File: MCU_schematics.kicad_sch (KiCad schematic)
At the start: 39 parts, among them Q1 SS8050, Q2 SS8050, U7 CH340C

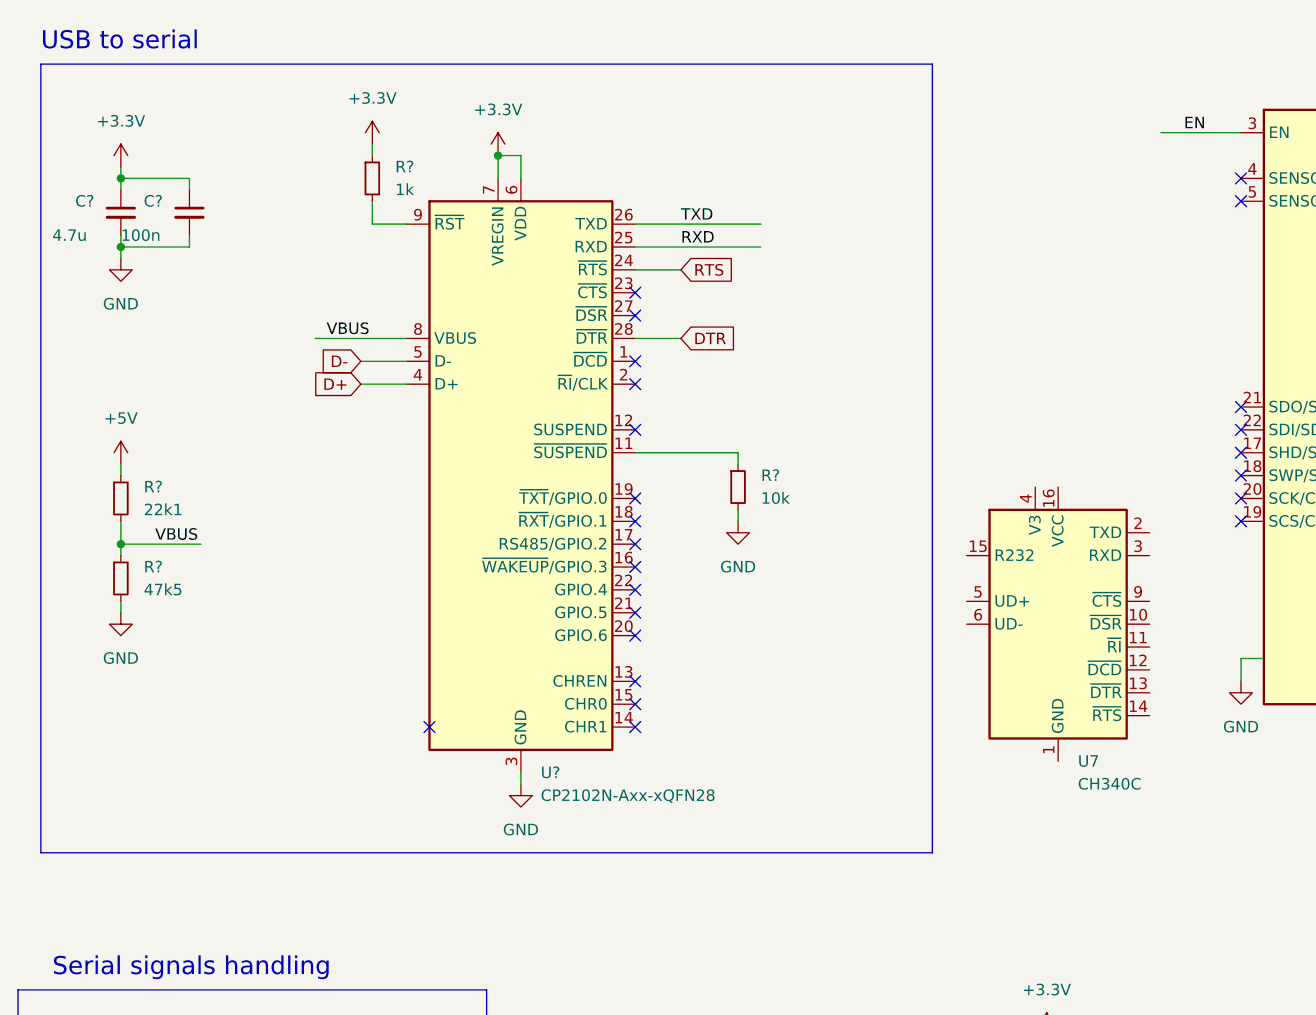
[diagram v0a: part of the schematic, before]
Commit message: version 1.1
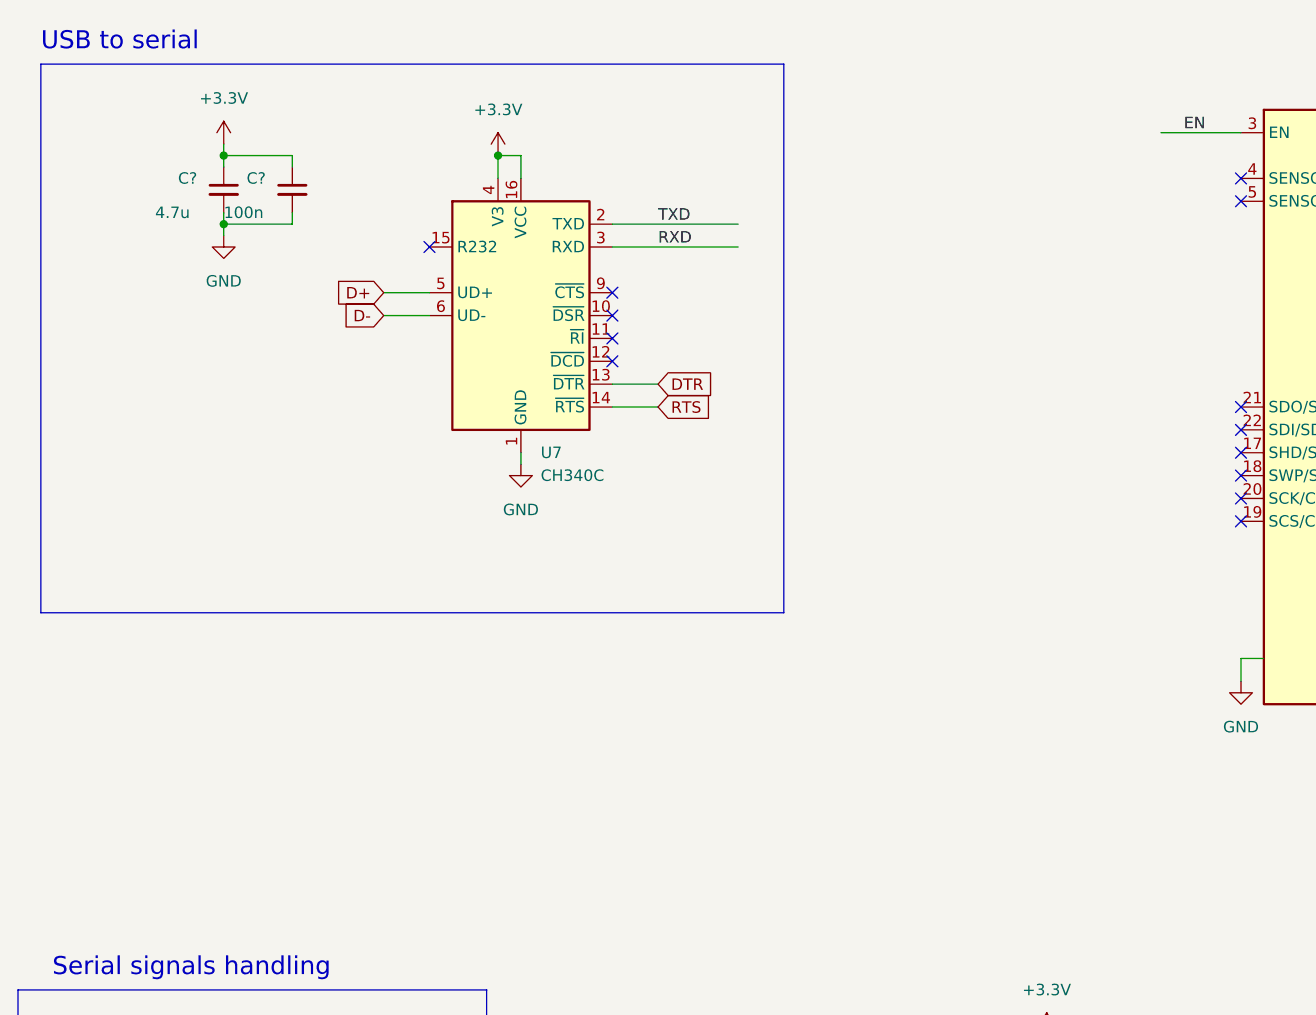
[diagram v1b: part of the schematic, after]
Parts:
- removed R?: 47k5, Resistor_SMD:R_0603_1608Metric_Pad0.98x0.95mm_HandSolder, symbol Device:R_Small
- removed R?: 1k, Resistor_SMD:R_0603_1608Metric_Pad0.98x0.95mm_HandSolder, symbol Device:R_Small
- removed R?: 10k, Resistor_SMD:R_0603_1608Metric_Pad0.98x0.95mm_HandSolder, symbol Device:R_Small
- removed R?: 22k1, Resistor_SMD:R_0603_1608Metric_Pad0.98x0.95mm_HandSolder, symbol Device:R_Small
- removed U?: CP2102N-Axx-xQFN28, Package_DFN_QFN:QFN-28-1EP_5x5mm_P0.5mm_EP3.35x3.35mm, symbol Interface_USB:CP2102N-Axx-xQFN28
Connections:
- net +3.3V: now also U7.16 (VCC), U7.4 (V3)
- net D+: now also U7.5 (UD+)
- net D-: now also U7.6 (UD-)
- net DTR: now also U7.13 (~{DTR})
- net GND: now also U7.1 (GND)
- net RTS: now also U7.14 (~{RTS})
- net RXD: now also U7.3 (RXD)
- net TXD: now also U7.2 (TXD)
- no-connect marks 28 -> 17
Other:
- moved on the sheet: C?, U7
